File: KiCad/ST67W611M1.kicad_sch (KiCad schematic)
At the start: 1 part, among them U201 ST67W611

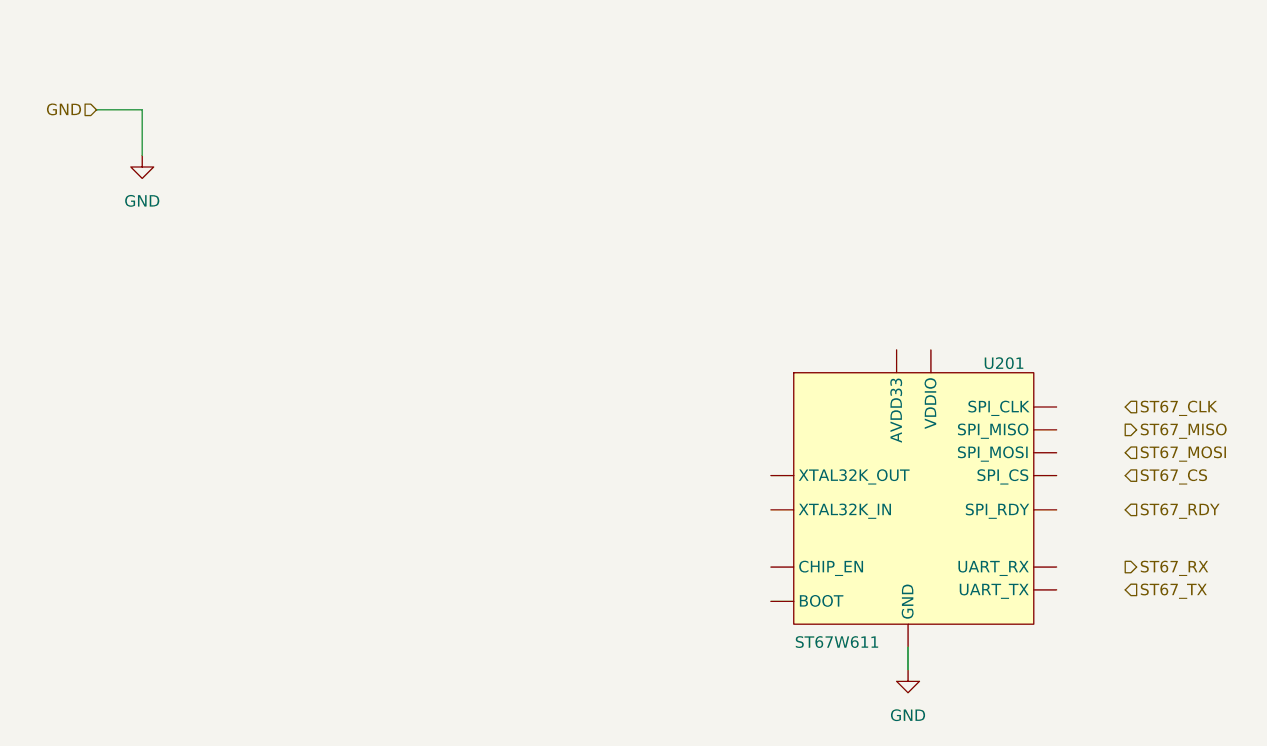
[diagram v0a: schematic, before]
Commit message: KiCad work
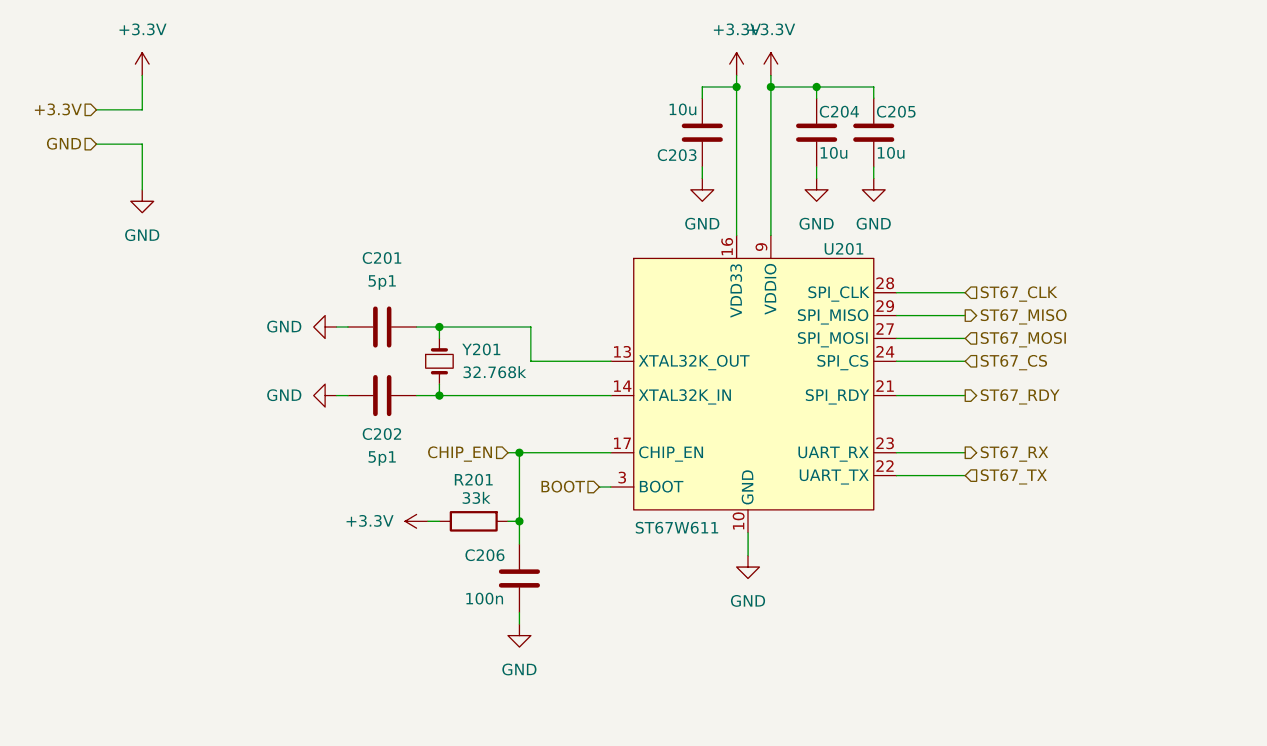
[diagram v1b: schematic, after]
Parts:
- added C201, C202: 5p1, symbol Device:C
- added C203, C204, C205: 10u, symbol Device:C
- added C206: 100n, symbol Device:C
- added R201: 33k, symbol Device:R
- added Y201: 32.768k, symbol Device:Crystal_Small
- U201: footprint (none) -> JPComms:ST67W611M1
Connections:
- net GND: now also U201.10 (GND), U201.15 (GND), U201.18 (GND), U201.26 (GND), U201.30 (GND), U201.32 (GND), C201.1, C202.1, C203.1, C204.2, C205.2, C206.1; no longer U201. (UART_TX)
- net ST67_CLK: now also U201.28 (SPI_CLK)
- net ST67_CS: now also U201.24 (SPI_CS)
- net ST67_MISO: now also U201.29 (SPI_MISO)
- net ST67_MOSI: now also U201.27 (SPI_MOSI)
- net ST67_RDY: now also U201.21 (SPI_RDY)
- net ST67_RX: now also U201.23 (UART_RX)
- net ST67_TX: now also U201.22 (UART_TX)
- new net: C201.2, U201.13 (XTAL32K_OUT), Y201.1
- new net: C202.2, U201.14 (XTAL32K_IN), Y201.2
- new net +3.3V: C203.2, C204.1, C205.1, R201.1, U201.16 (VDD33), U201.25 (VDDIO), U201.9 (VDDIO)
- new net BOOT: U201.3 (BOOT)
- new net CHIP_EN: C206.2, R201.2, U201.17 (CHIP_EN)
